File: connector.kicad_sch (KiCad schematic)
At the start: 2 parts, among them J401 AXK500137YG, J402 AXK500137YG

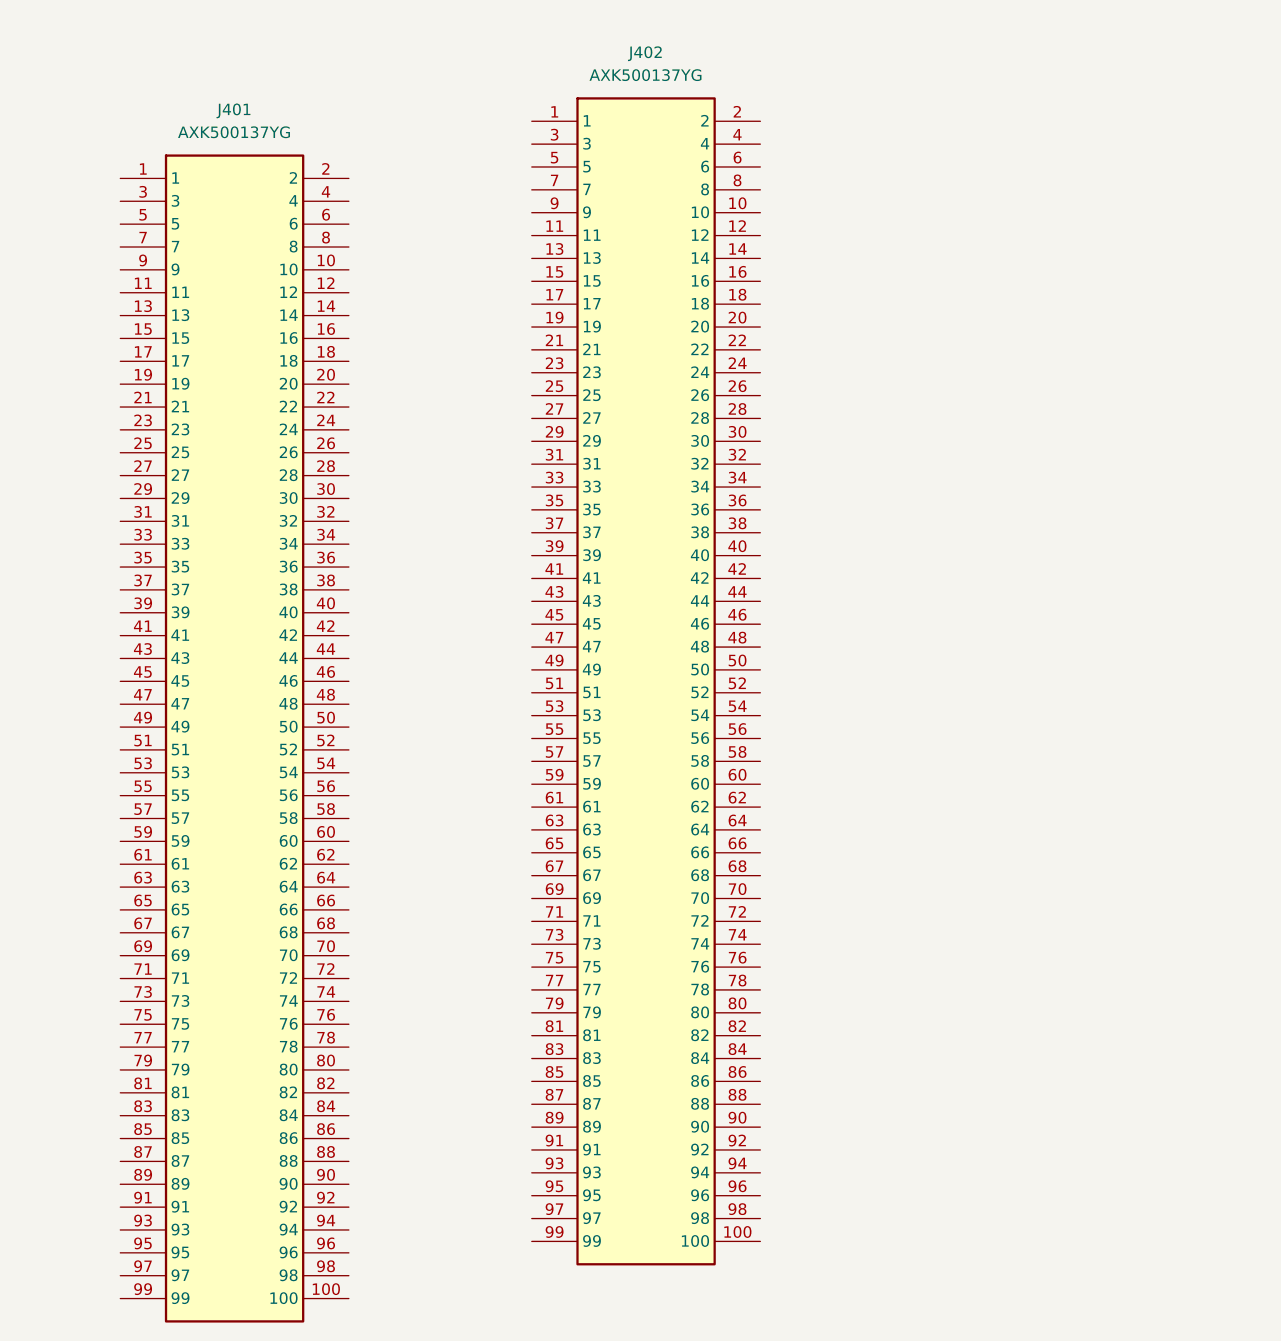
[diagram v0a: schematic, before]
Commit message: feat: continue improve sch design
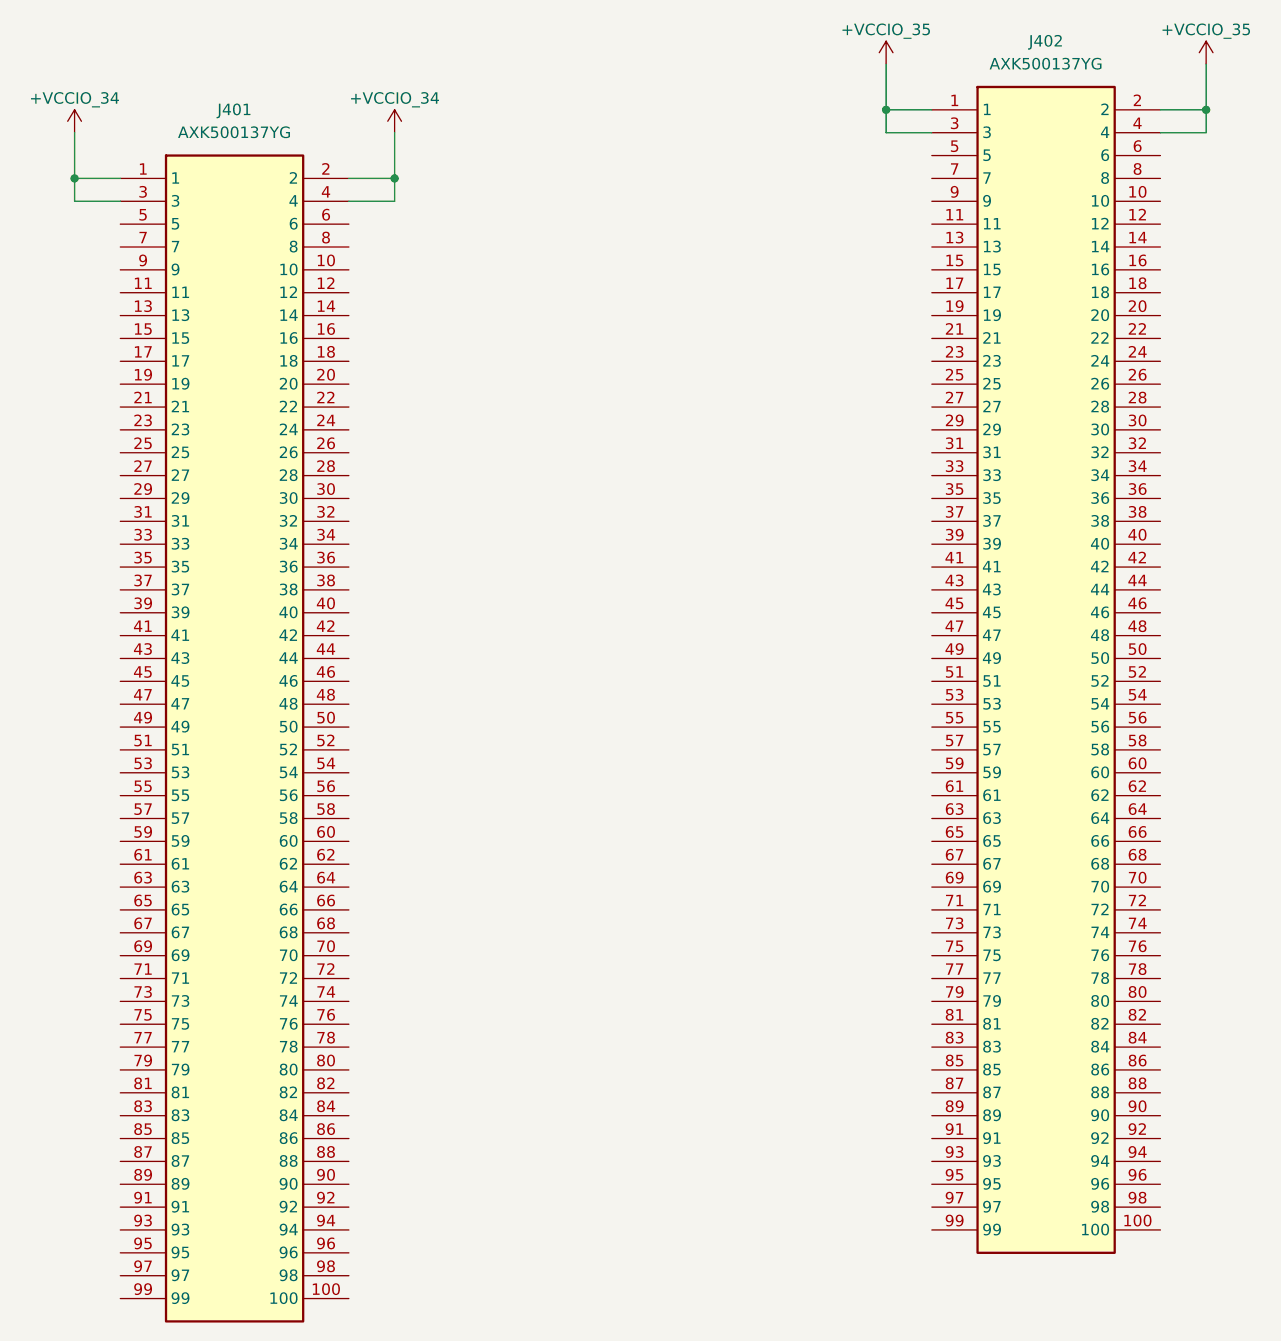
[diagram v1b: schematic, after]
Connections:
- net +VCCIO_35: now reaches J402.1
- net +VCCIO_35: now also J402.2, J402.3, J402.4
- net +VCCIO_34: now reaches J401.1
- net +VCCIO_34: now also J401.2, J401.3, J401.4
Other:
- moved on the sheet: J402
